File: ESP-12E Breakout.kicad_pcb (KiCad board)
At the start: 2 copper layers, 40 x 40 mm, 6 parts, among them J3 Conn_01x08_Pin, J4 Conn_01x08_Pin, J5 Conn_01x06_Pin, U1 ESP-12E

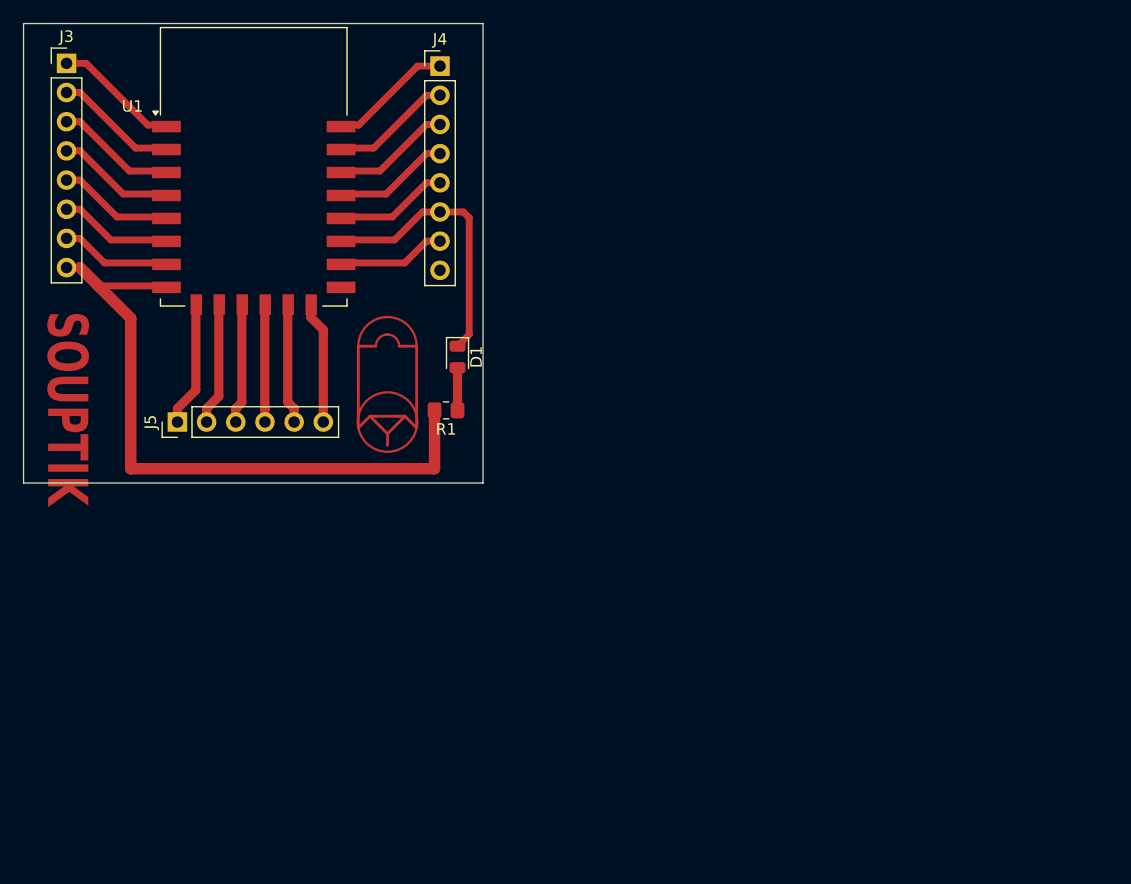
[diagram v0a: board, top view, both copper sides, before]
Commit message: Add files via upload
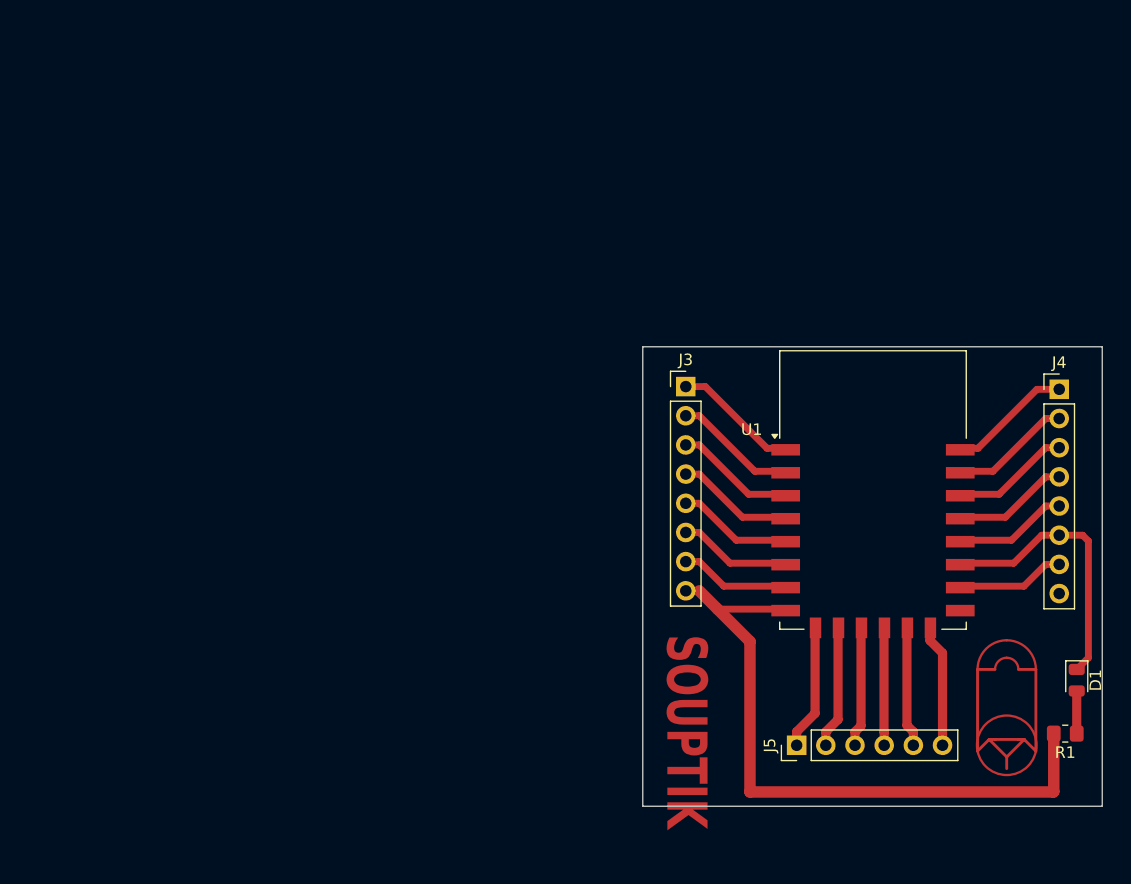
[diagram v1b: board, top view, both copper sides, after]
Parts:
- moved J5 60.8 mm to (160.5, 110.3)
- moved U1 60.8 mm to (167.2, 88.1)
- moved D1 60.8 mm to (184.9, 104.6)
- moved J3 60.8 mm to (150.9, 79.1)
- moved J4 60.8 mm to (183.4, 79.3)
- moved R1 60.8 mm to (183.9, 109.3)
